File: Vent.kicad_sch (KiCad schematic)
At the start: 11 parts, among them J2 B2B-XH-A_LF__SN_, J3 Conn_01x03_Pin, SW1 SW_Push, U1 ESP32-H2-MINI-1-H2

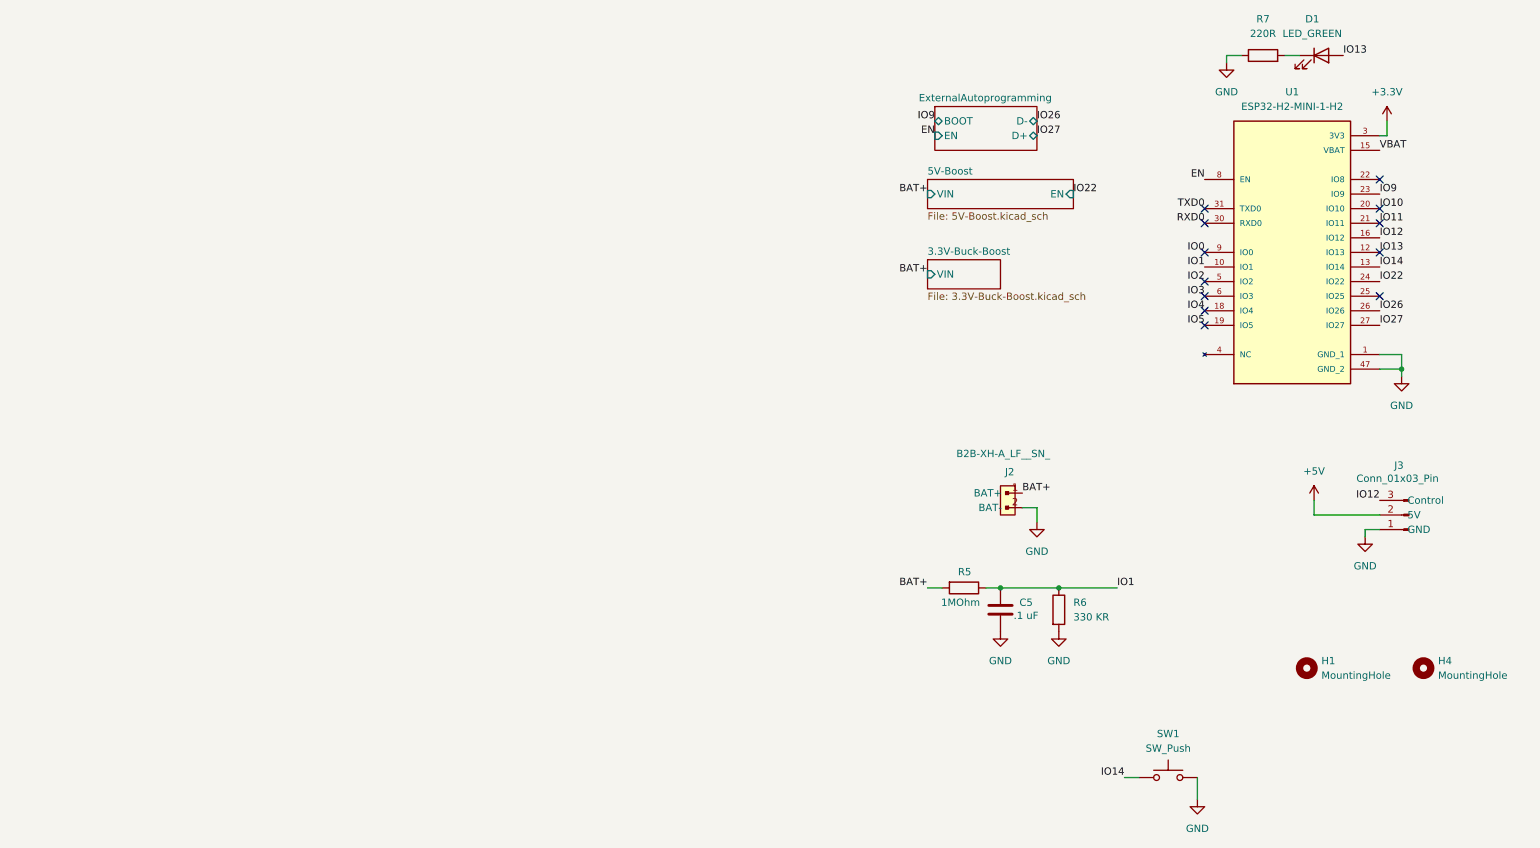
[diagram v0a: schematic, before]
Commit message: Schematic Organization
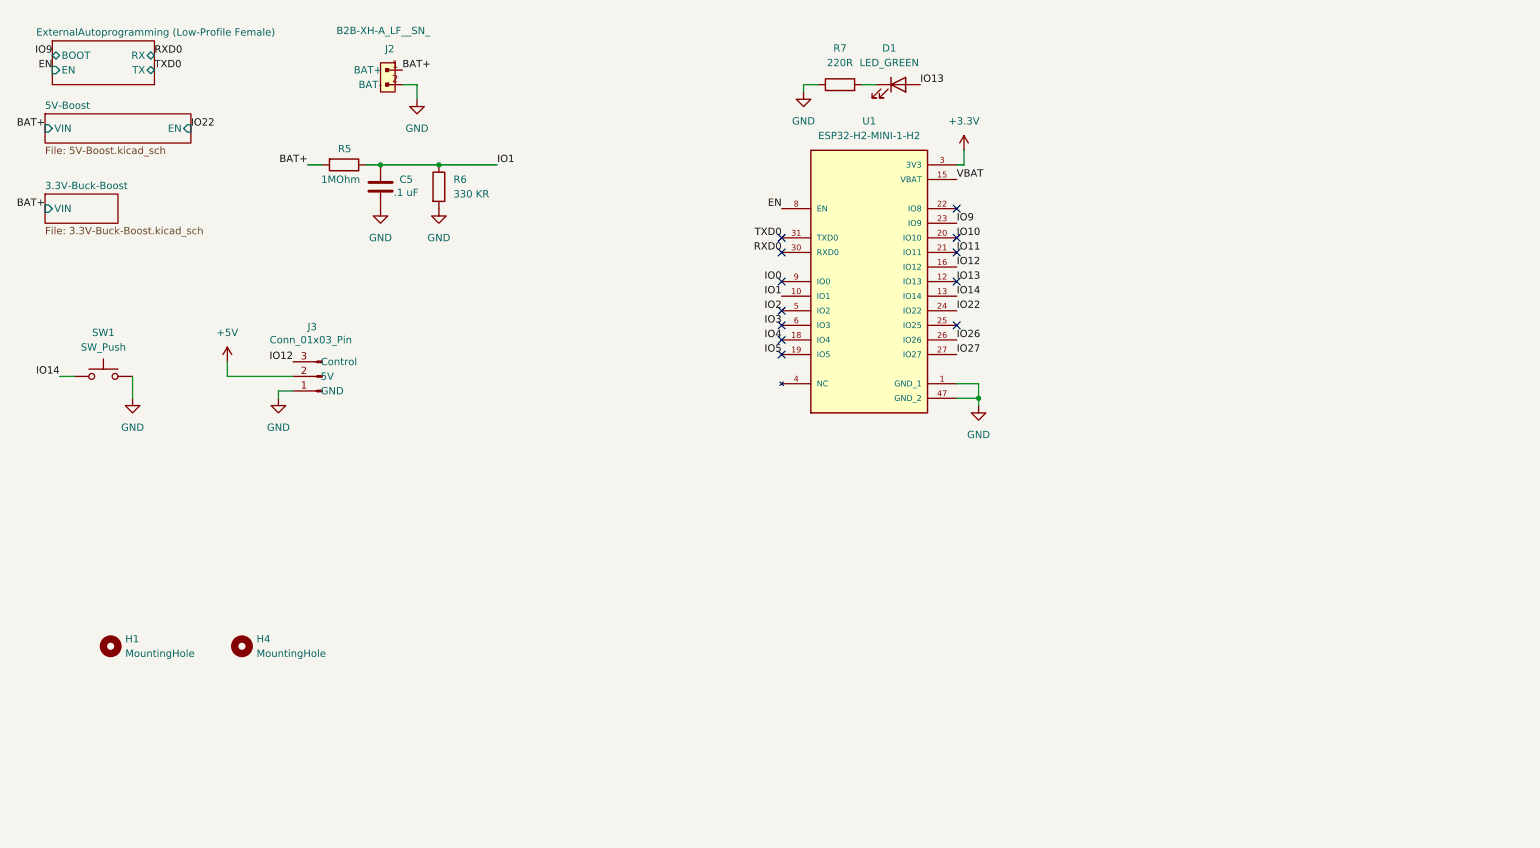
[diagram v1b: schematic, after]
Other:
- sheet ExternalAutoprogramming renamed ExternalAutoprogramming (Low-Profile Female)
- sheet ExternalAutoprogramming (Low-Profile Female) ports: added RX, TX; removed D+, D-
- moved on the sheet: C5, D1, H1, H4, J2, J3, R5, R6, R7, SW1, U1
